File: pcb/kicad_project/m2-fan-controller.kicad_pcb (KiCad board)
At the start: 2 copper layers, 22 x 30 mm, 18 parts, among them J1 Bus_M.2_Socket_E, J2 Conn_01x04, J3 Conn_01x04, J4 JST PH_S2B-PH-K, J5 Conn_02x02_Odd_Even, U1 STM32F042F6P6

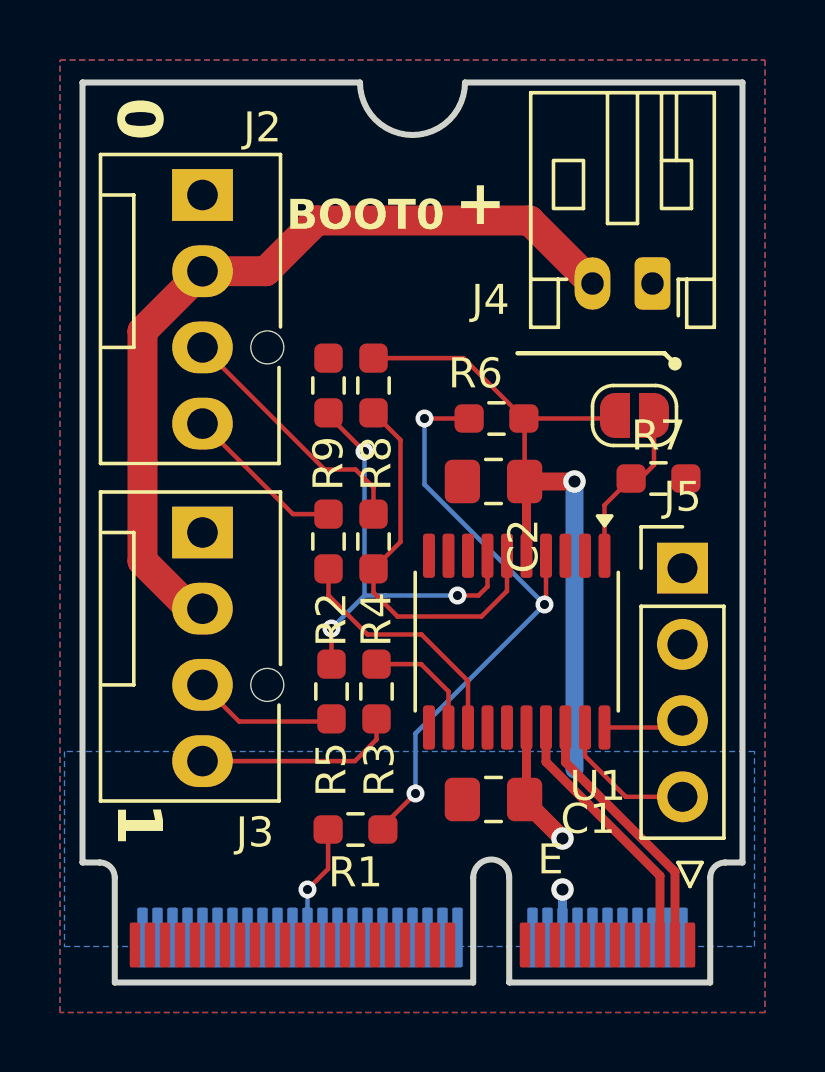
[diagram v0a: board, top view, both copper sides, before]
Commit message: Final revision
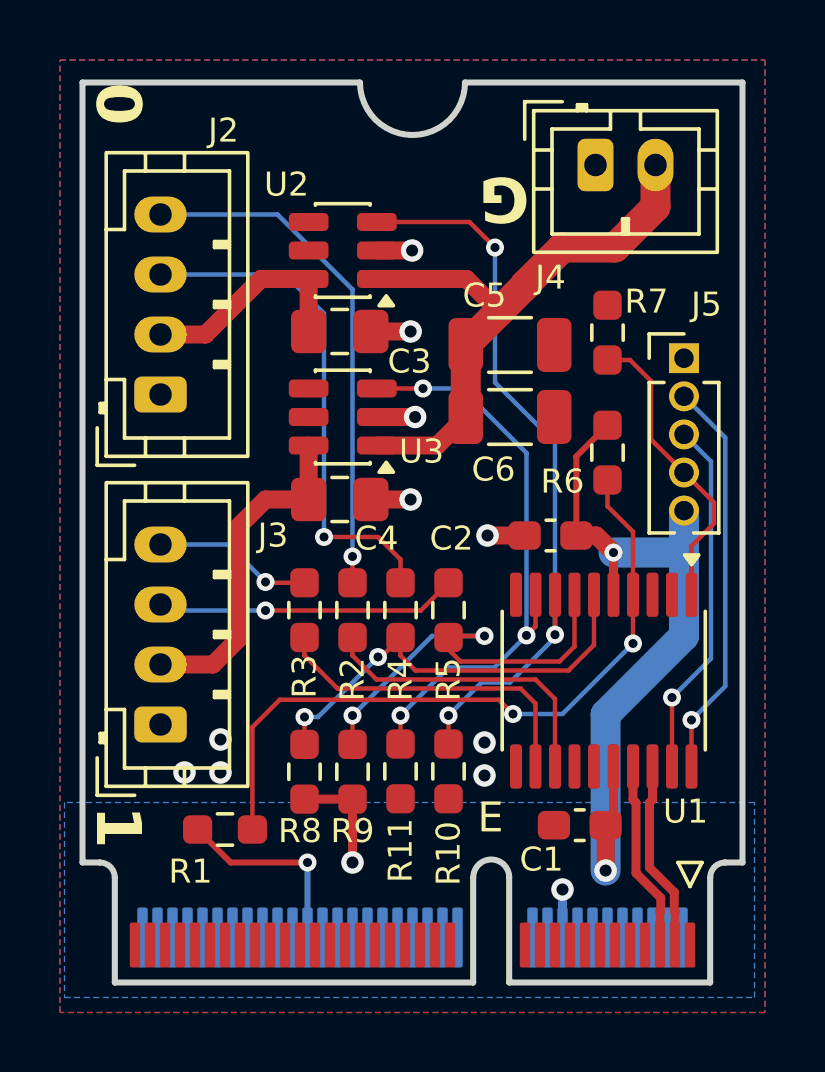
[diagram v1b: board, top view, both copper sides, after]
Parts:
- removed JP1: Jumper_2_Open, Jumper:SolderJumper-2_P1.3mm_Open_RoundedPad1.0x1.5mm
- added C3: 0.1uF, Capacitor_SMD:C_0805_2012Metric_Pad1.18x1.45mm_HandSolder, F.Cu at (136.6, 88.3)
- added C4: 0.1uF, Capacitor_SMD:C_0805_2012Metric_Pad1.18x1.45mm_HandSolder, F.Cu at (136.6, 93.9)
- added C5: 1uF, Capacitor_SMD:C_1206_3216Metric, F.Cu at (142.2, 88.8)
- added C6: 1uF, Capacitor_SMD:C_1206_3216Metric, F.Cu at (142.2, 91.2)
- added R10: 10kOhm, Resistor_SMD:R_0603_1608Metric_Pad0.98x0.95mm_HandSolder, F.Cu at (140.2, 103.0)
- added R11: 10kOhm, Resistor_SMD:R_0603_1608Metric_Pad0.98x0.95mm_HandSolder, F.Cu at (138.6, 103.0)
- added U2: TPS22810DBV, Package_TO_SOT_SMD:SOT-23-6, F.Cu at (136.7, 85.6)
- added U3: TPS22810DBV, Package_TO_SOT_SMD:SOT-23-6, F.Cu at (136.7, 91.2)
- C1, C2: footprint Capacitor_SMD:C_0805_2012Metric_Pad1.18x1.45mm_HandSolder -> Capacitor_SMD:C_0603_1608Metric_Pad1.08x0.95mm_HandSolder
- J2, J3: value Conn_01x04 -> JST PH_B4B-PH-K; footprint Connector:FanPinHeader_1x04_P2.54mm_Vertical -> Connector_JST:JST_PH_B4B-PH-K_1x04_P2.00mm_Vertical
- J4: footprint Connector_JST:JST_PH_S2B-PH-K_1x02_P2.00mm_Horizontal -> Connector_JST:JST_PH_B2B-PH-K_1x02_P2.00mm_Vertical
- J5: footprint Connector_PinHeader_2.54mm:PinHeader_1x04_P2.54mm_Vertical -> Connector_PinHeader_1.27mm:PinHeader_1x05_P1.27mm_Vertical
- moved R8 13.1 mm to (135.4, 103.0), turned to 90 degrees
- moved R9 12.9 mm to (137.0, 103.0), turned to 90 degrees
- moved J5 7.00 mm to (148.1, 89.2)
- moved J2 6.80 mm to (130.6, 90.4), turned to 90 degrees
- moved J3 6.55 mm to (130.6, 101.4), turned to 90 degrees
- moved R7 5.15 mm to (145.5, 88.3), turned to 90 degrees
- moved R5 4.75 mm to (140.2, 97.6), turned to 90 degrees
- moved J4 4.38 mm to (145.1, 82.8), turned to 0 degrees
- moved R1 4.35 mm to (132.8, 104.9)
- moved R6 3.87 mm to (145.5, 92.3), turned to -90 degrees
- moved R3 3.62 mm to (135.4, 97.6), turned to 90 degrees
- moved U1 3.18 mm to (145.4, 99.9)
- moved C1 3.00 mm to (144.6, 104.8)
- moved C2 2.62 mm to (143.6, 95.1)
- moved R4 2.46 mm to (138.6, 97.6)
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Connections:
- J2 pad 2: +12V -> Net-(J2-Pin_2)
- J3 pad 2: +12V -> Net-(J3-Pin_2)
- J5 pad 2: +3.3V -> SWCLK
- J5 pad 3: SWCLK -> SWDIO
- J5 pad 4: SWDIO -> BOOT0
- U1 pad 8: unconnected-(U1-PA2-Pad8) -> EN_0
- U1 pad 9: unconnected-(U1-PA3-Pad9) -> EN_1
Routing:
- net EN_0: track 0.00 -> 24.8 mm, vias 0 -> 3
- net EN_1: track 0.00 -> 19.4 mm, vias 0 -> 3
- net Net-(J2-Pin_4): track 5.45 -> 17.2 mm, vias 0 -> 1
- net Net-(J3-Pin_2): track 0.00 -> 11.2 mm
- net SWCLK: track 2.70 -> 13.4 mm, vias 0 -> 1
- net Net-(J2-Pin_3): track 8.55 -> 17.1 mm, vias 0 -> 1
- net +12V: track 27.6 -> 19.9 mm
- net Net-(J2-Pin_2): track 0.00 -> 7.45 mm
- net SWDIO: track 4.76 -> 12.0 mm, vias 0 -> 1
- net PWM_1: track 3.98 -> 11.1 mm
- net GND: track 1.60 -> 7.94 mm, vias 1 -> 11
- net Net-(J3-Pin_3): track 4.31 -> 10.1 mm, vias 0 -> 1
- net BOOT0: track 5.94 -> 10.0 mm
- net Net-(J1-~{PERST0}): track 3.88 -> 6.62 mm
- net USB_D-: track 8.82 -> 6.34 mm
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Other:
- board text added: "12V"
- board text added: "3.3V"
- board text added: "G"
- board text added: "GND"
- board text added: "PCB thickness 0.8 mm"
- board text added: "PWM"
- board text added: "SWCLK"
- board text added: "SWDIO"
- board text added: "TACH"
- board text removed: "+"
- board text removed: "M.2 fan controller"
